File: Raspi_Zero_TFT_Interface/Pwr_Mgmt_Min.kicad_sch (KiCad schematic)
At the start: 19 parts, among them Q4 SSM3J358R, SW2 Rocker Switch SPST, U11 MCP73831-2-OT, U13 LD39050

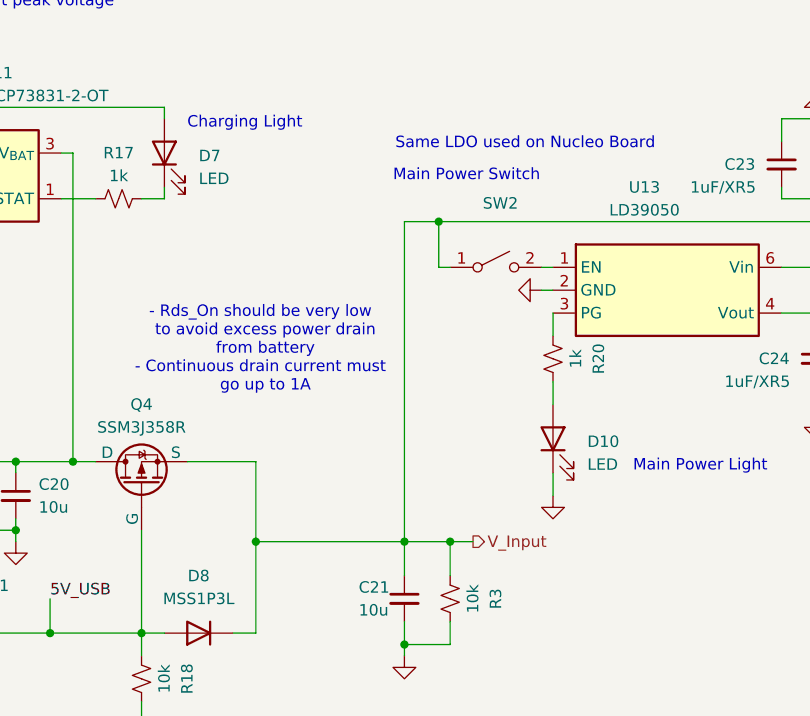
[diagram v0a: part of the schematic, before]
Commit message: Small change to Raspi Board
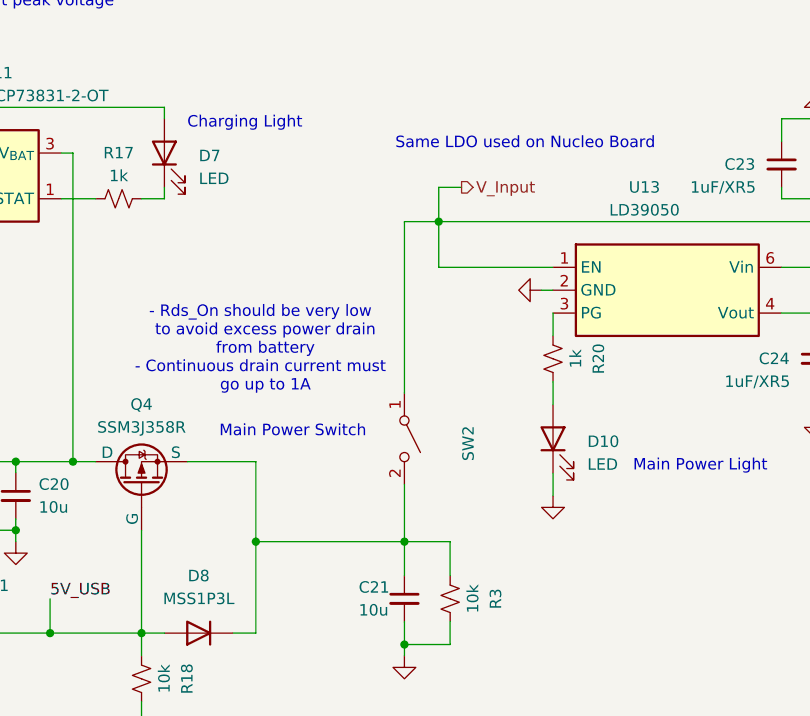
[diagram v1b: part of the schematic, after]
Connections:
- net V_Input: now also U13.1 (EN); no longer C21.1, D8.1 (K), Q4.2 (S), R3.1
- net at SW2.2 (B): now also C21.1, D8.1 (K), Q4.2 (S), R3.1; no longer U13.1 (EN)
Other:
- moved on the sheet: SW2
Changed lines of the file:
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@@
-	)
-	(junction
-		(at 144.78 83.82)
-		(diameter 0)
-		(color 0 0 0 0)
 	)
 	(junction
@@
 	(wire
 		(pts
+			(xy 139.7 77.47) (xy 139.7 83.82)
+		)
+		(stroke
+			(width 0)
+			(type default)
+		)
+	)
+	(wire
+		(pts
 			(xy 102.87 40.64) (xy 102.87 74.93)
 		)
@@
 	(wire
 		(pts
-			(xy 139.7 48.26) (xy 139.7 83.82)
+			(xy 139.7 48.26) (xy 139.7 67.31)
 		)
 		(stroke
@@
 	(wire
 		(pts
-			(xy 144.78 53.34) (xy 143.51 53.34)
+			(xy 143.51 53.34) (xy 156.21 53.34)
 		)
 		(stroke
@@
 	(wire
 		(pts
+			(xy 143.51 44.45) (xy 143.51 48.26)
+		)
+		(stroke
+			(width 0)
+			(type default)
+		)
+	)
+	(wire
+		(pts
 			(xy 123.19 93.98) (xy 120.65 93.98)
 		)
@@
 	(wire
 		(pts
-			(xy 144.78 83.82) (xy 147.32 83.82)
-		)
-		(stroke
-			(width 0)
-			(type default)
-		)
-	)
-	(wire
-		(pts
 			(xy 154.94 55.88) (xy 156.21 55.88)
 		)
@@
 	(wire
 		(pts
-			(xy 156.21 53.34) (xy 154.94 53.34)
-		)
-		(stroke
-			(width 0)
-			(type default)
-		)
-	)
-	(wire
-		(pts
 			(xy 74.93 34.29) (xy 74.93 35.56)
 		)
@@
 	(wire
 		(pts
+			(xy 146.05 44.45) (xy 143.51 44.45)
+		)
+		(stroke
+			(width 0)
+			(type default)
+		)
+	)
+	(wire
+		(pts
 			(xy 144.78 92.71) (xy 144.78 95.25)
 		)
@@
 	(text "Main Power Switch"
 		(exclude_from_sim no)
-		(at 138.43 43.942 0)
+		(at 119.126 72.39 0)
 		(effects
 			(font
@@
 	(hierarchical_label "V_Input"
 		(shape output)
-		(at 147.32 83.82 0)
+		(at 146.05 44.45 0)
 		(fields_autoplaced yes)
 		(effects
@@
 	(symbol
 		(lib_id "Switch:SW_SPST")
-		(at 149.86 53.34 0)
+		(at 139.7 72.39 270)
 		(unit 1)
 		(exclude_from_sim no)
@@
 		(dnp no)
 		(property "Reference" "SW2"
-			(at 150.368 46.228 0)
+			(at 146.812 72.898 0)
 			(effects
 				(font
@@
 		)
 		(property "Value" "Rocker Switch SPST"
-			(at 149.86 49.53 0)
+			(at 143.51 72.39 0)
 			(effects
 				(font
@@
 		)
 		(property "Footprint" "Connector_PinHeader_2.54mm:PinHeader_1x02_P2.54mm_Vertical"
-			(at 149.86 53.34 0)
+			(at 139.7 72.39 0)
 			(effects
 				(font
@@
 		)
 		(property "Datasheet" "~"
-			(at 149.86 53.34 0)
+			(at 139.7 72.39 0)
 			(effects
 				(font
@@
 		)
 		(property "Description" ""
-			(at 149.86 53.34 0)
-			(effects
-				(font
+			(at 139.7 72.39 0)
+			(effects
+				(font

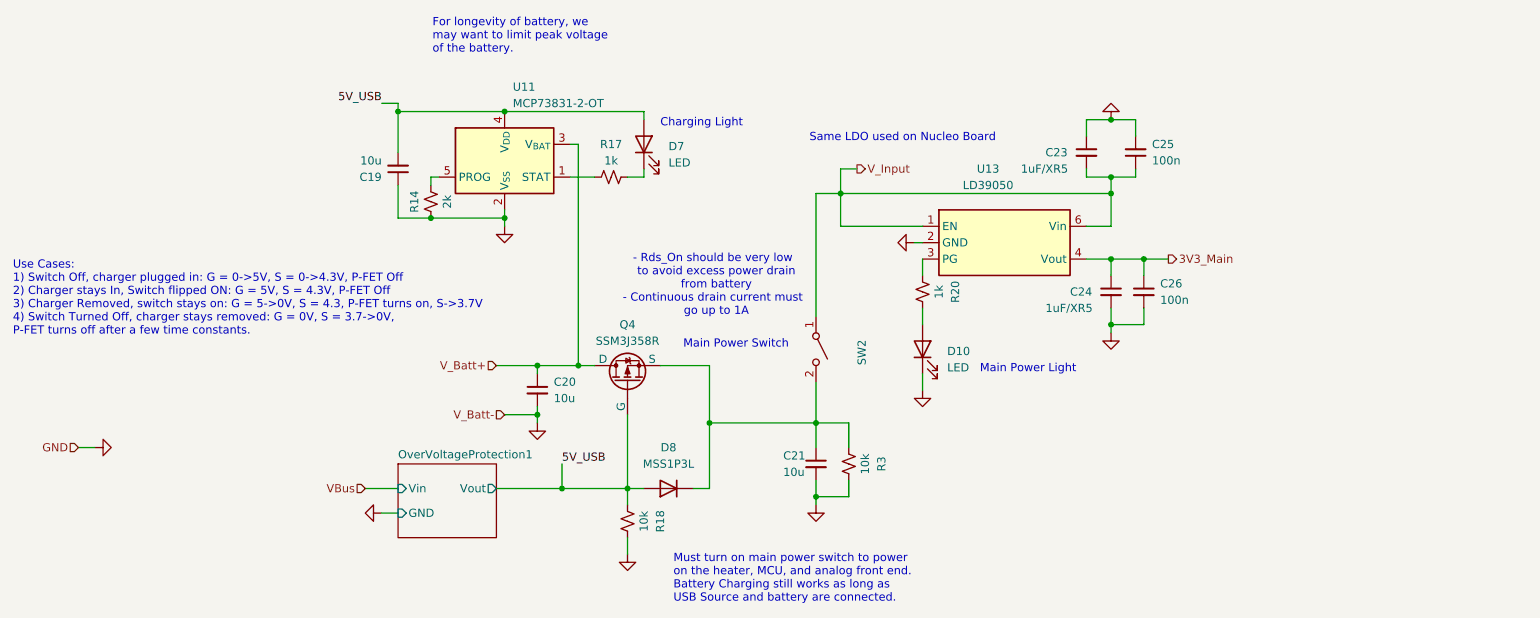
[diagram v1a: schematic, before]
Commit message: Nearly Finalized Boards
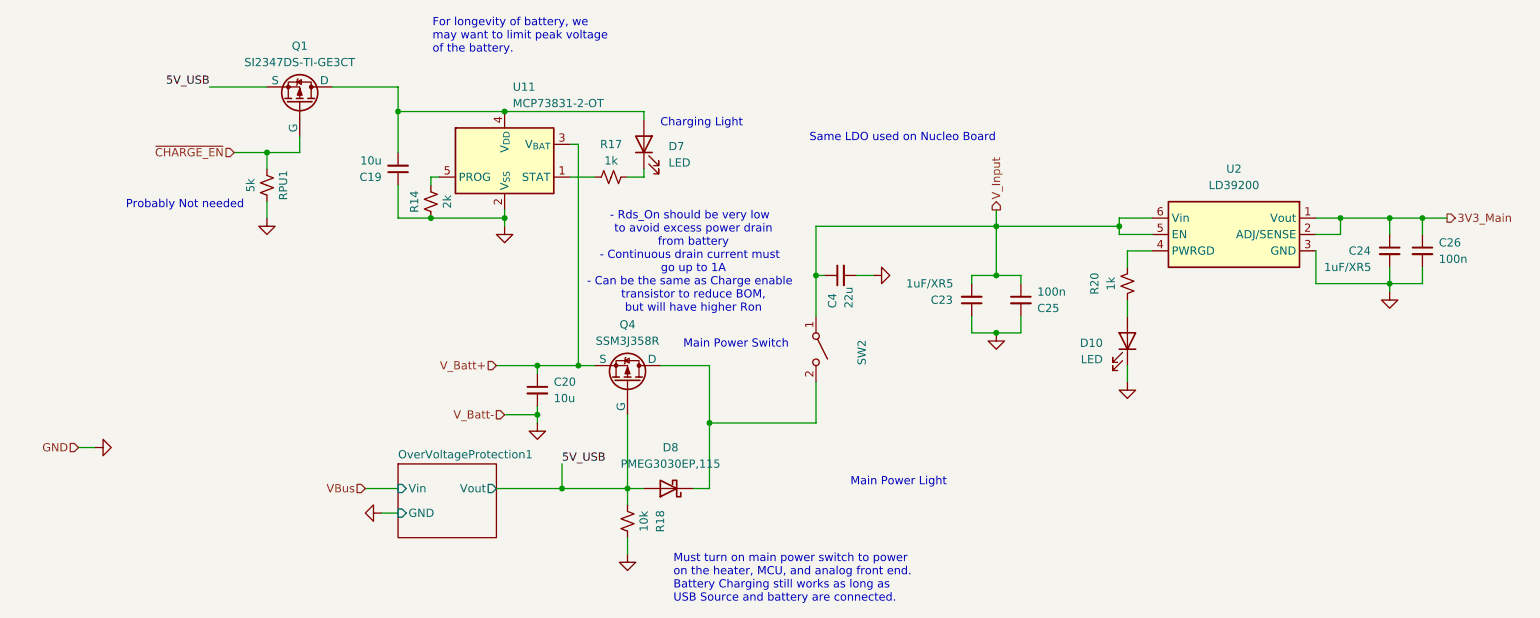
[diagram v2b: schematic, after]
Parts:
- removed C21: 10u, Capacitor_SMD:C_0603_1608Metric_Pad1.08x0.95mm_HandSolder, symbol Device:C_Small
- removed R3: 10k, Resistor_SMD:R_0603_1608Metric_Pad0.98x0.95mm_HandSolder, symbol Device:R_Small_US
- removed U13: LD39050, Package_DFN_QFN:DFN-6-1EP_3x3mm_P0.95mm_EP1.7x2.6mm, symbol FrontEndPrototype_Rev1-rescue:LD39050
- added C4: 22u, Capacitor_SMD:C_0603_1608Metric_Pad1.08x0.95mm_HandSolder, symbol Device:C_Small
- added Q1: SI2347DS-TI-GE3CT, Package_TO_SOT_SMD:SOT-23-3, symbol FrontEndPrototype_Rev1-rescue:SSM3J358R
- added RPU1: 5k, Resistor_SMD:R_0603_1608Metric_Pad0.98x0.95mm_HandSolder, symbol Device:R_Small_US
- added U2: LD39200, Package_DFN_QFN:DFN-6-1EP_3x3mm_P0.95mm_EP1.7x2.6mm, symbol FrontEndPrototype_Rev1-rescue:LD39200_Fixed
- D8: value MSS1P3L -> PMEG3030EP,115; footprint Diode_SMD:D_MicroSMP_AK -> Diode_SMD:D_SOD-128; symbol Device:D -> Device:D_Schottky
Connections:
- net 3V3_Main: now also U2.1 (Vout), U2.2 (ADJ/SENSE)
- net 5V_USB: now also Q1.2 (S); no longer C19.2, D7.2 (A), U11.4 (V_{DD})
- net GND: now also C4.2, RPU1.2, U2.3 (GND)
- net V_Batt+: now also Q4.2 (S); no longer Q4.3 (D)
- net V_Input: now also C4.1, U2.5 (EN), U2.6 (Vin)
- net at D8.1 (K), SW2.2 (B): now also Q4.3 (D); no longer Q4.2 (S)
- net at R20.1: now also U2.4 (PWRGD)
- new net: C19.2, D7.2 (A), Q1.3 (D), U11.4 (V_{DD})
- new net ~{CHARGE_EN}: Q1.1 (G), RPU1.1
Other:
- note added: "- Rds_On should be very low to avoid excess power drain from battery - Continuous drain current must go up to 1A - Can be the same as Charge enable transistor to reduce BOM, but will have higher Ron"
- note added: "Probably Not needed"
- note removed: "- Rds_On should be very low to avoid excess power drain from battery - Continuous drain current must go up to 1A"
- note removed: "Use Cases: 1) Switch Off, charger plugged in: G = 0->5V, S = 0->4.3V, P-FET Off 2) Charger stays In, Switch flipped ON: G = 5V, S = 4.3V, P-FET Off 3) Charger Removed, switch stays on: G = 5->0V, S = 4.3, P-FET turns on, S->3.7V 4) Switch Turned Off, charger stays removed: G = 0V, S = 3.7->0V, P-FET turns off after a few time constants."
- moved on the sheet: C23, C24, C25, C26, D10, Q4, R20
